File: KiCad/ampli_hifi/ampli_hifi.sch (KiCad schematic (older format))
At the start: 7 parts, among them T101 Torique 2x9v

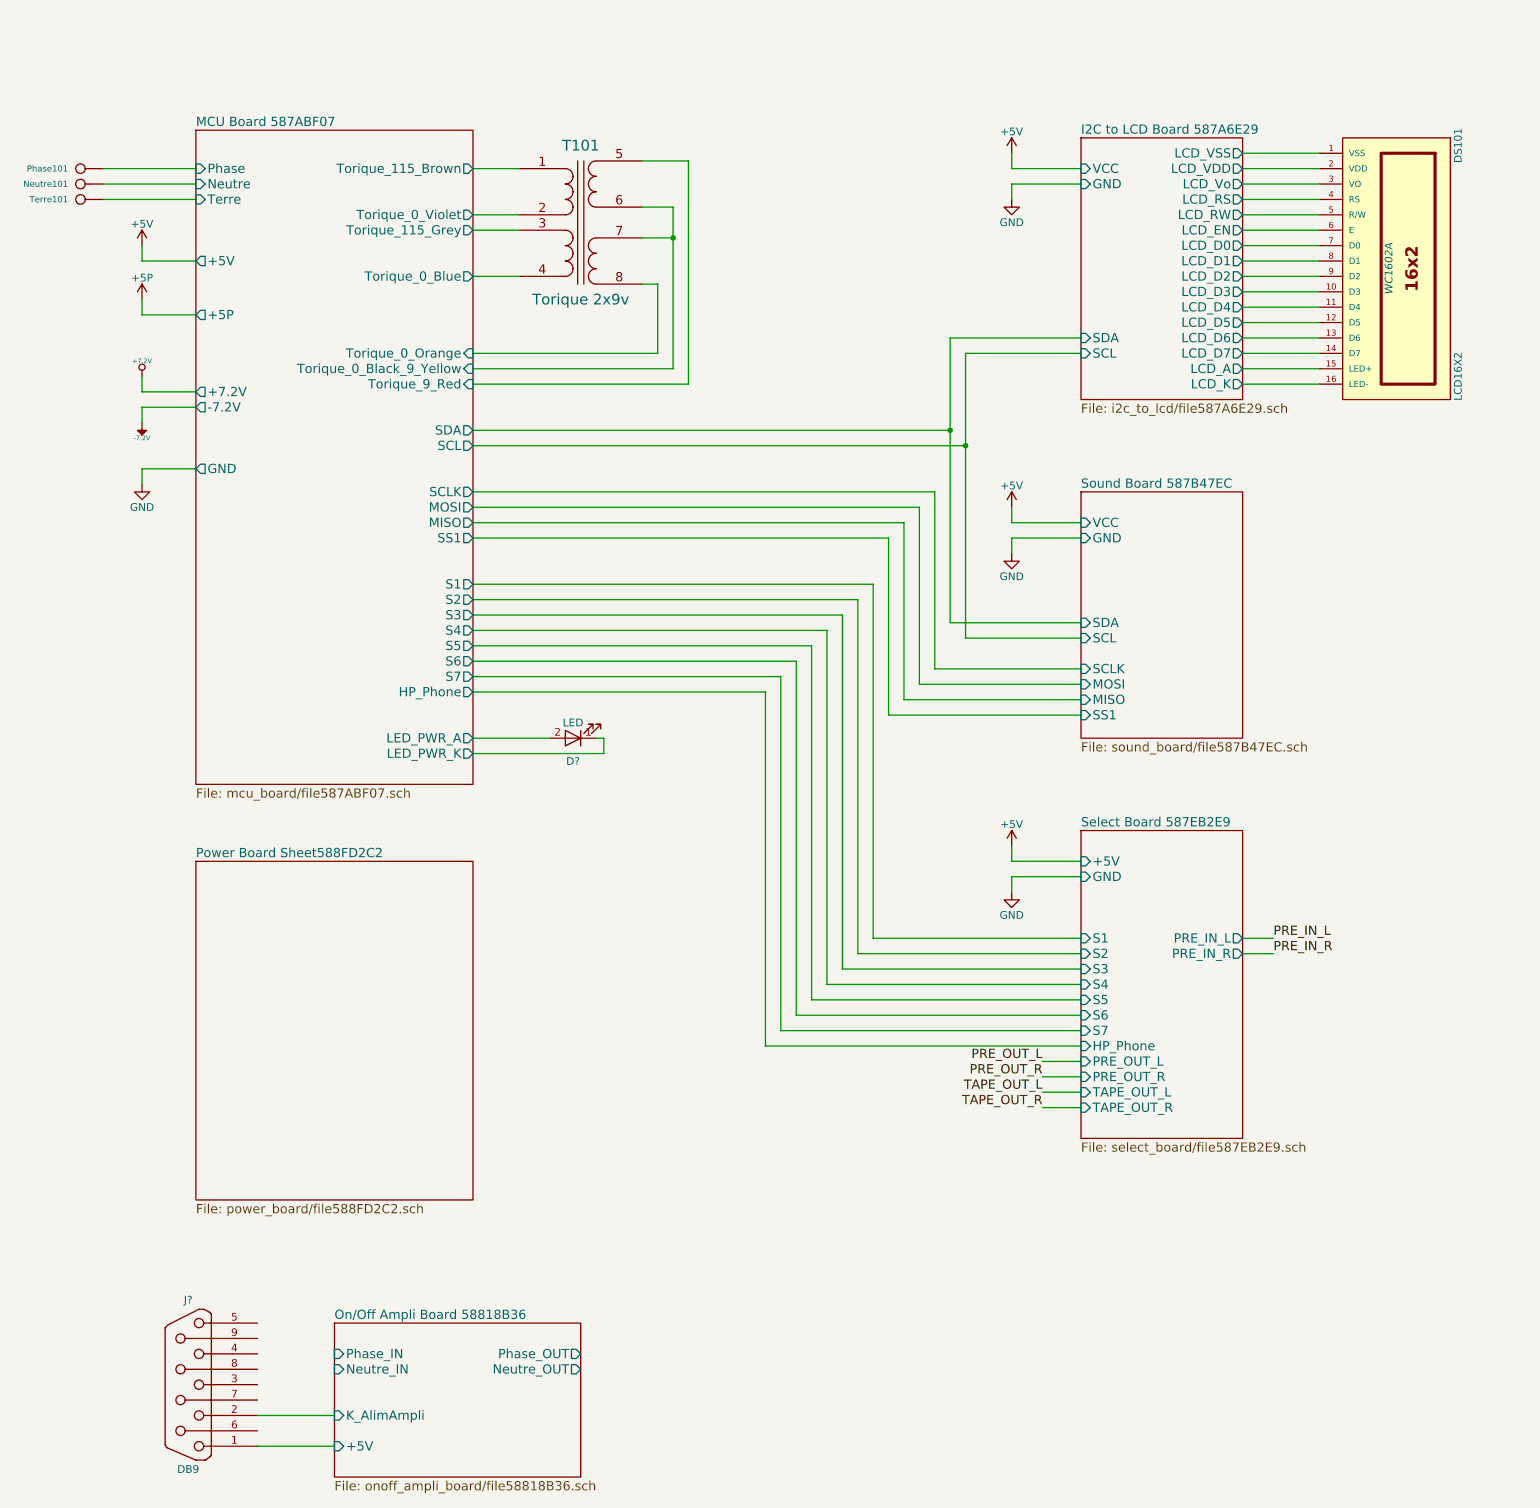
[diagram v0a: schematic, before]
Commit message: Divers
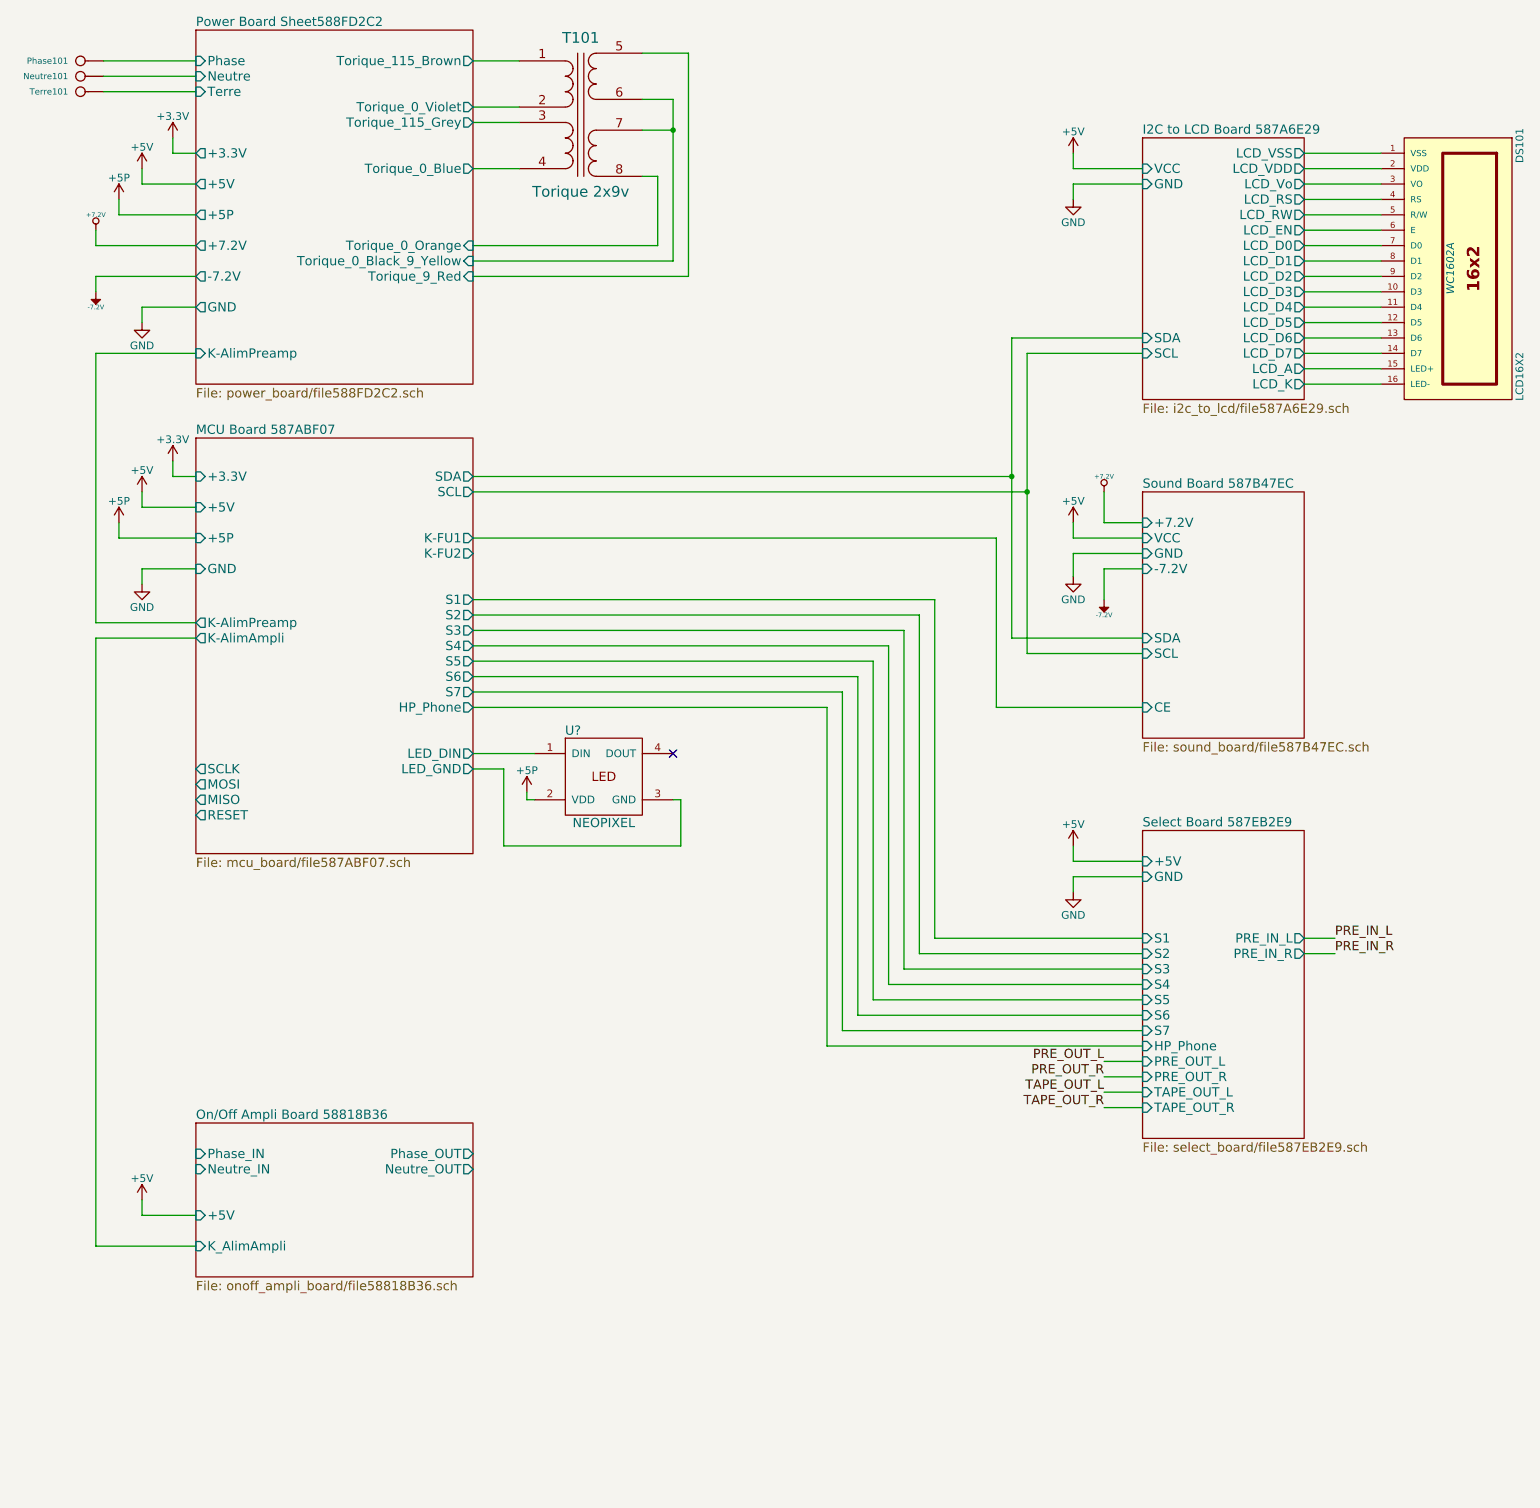
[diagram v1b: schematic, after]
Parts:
- removed D?: LED, symbol LED
- removed J?: DB9, symbol DB9
- added U?: NEOPIXEL, symbol NEOPIXEL
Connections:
- net +5P: now also U?.2 (VDD)
- net MCU Board 587ABF07/Neutre renamed Power Board Sheet588FD2C2/Neutre
- net MCU Board 587ABF07/Phase renamed Power Board Sheet588FD2C2/Phase
- net MCU Board 587ABF07/Terre renamed Power Board Sheet588FD2C2/Terre
- net MCU Board 587ABF07/Torique_0_Black_9_Yellow renamed Power Board Sheet588FD2C2/Torique_0_Black_9_Yellow
- net MCU Board 587ABF07/Torique_0_Blue renamed Power Board Sheet588FD2C2/Torique_0_Blue
- net MCU Board 587ABF07/Torique_0_Orange renamed Power Board Sheet588FD2C2/Torique_0_Orange
- net MCU Board 587ABF07/Torique_0_Violet renamed Power Board Sheet588FD2C2/Torique_0_Violet
- net MCU Board 587ABF07/Torique_115_Brown renamed Power Board Sheet588FD2C2/Torique_115_Brown
- net MCU Board 587ABF07/Torique_115_Grey renamed Power Board Sheet588FD2C2/Torique_115_Grey
- net MCU Board 587ABF07/Torique_9_Red renamed Power Board Sheet588FD2C2/Torique_9_Red
- new net MCU Board 587ABF07/LED_DIN: U?.1 (DIN)
- new net MCU Board 587ABF07/LED_GND: U?.3 (GND)
- no-connect marks 0 -> 1
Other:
- moved on the sheet: DS101, Neutre101, Phase101, T101, Terre101
